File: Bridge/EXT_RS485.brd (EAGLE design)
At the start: 22.5 x 72 mm, 17 parts, among them IC1 SN65HVD72D, X1 V1, X2 GND, X3 V2, X4 TERM, X5 TERM

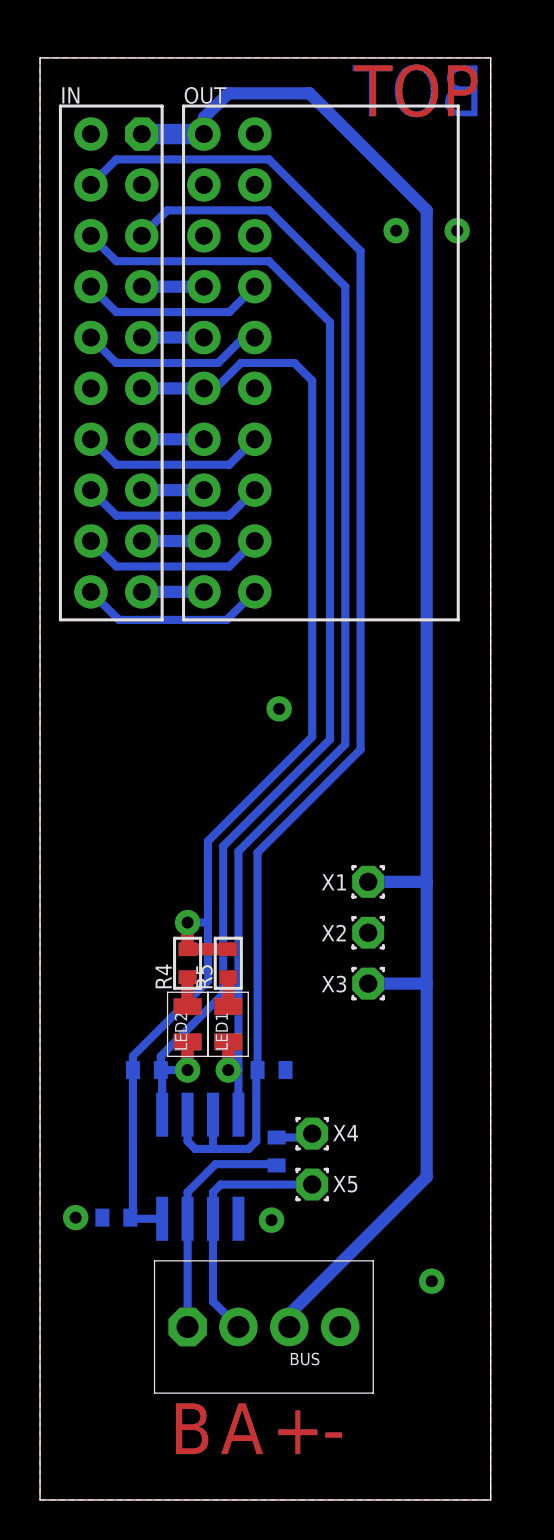
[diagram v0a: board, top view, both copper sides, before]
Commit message: Added S4M13
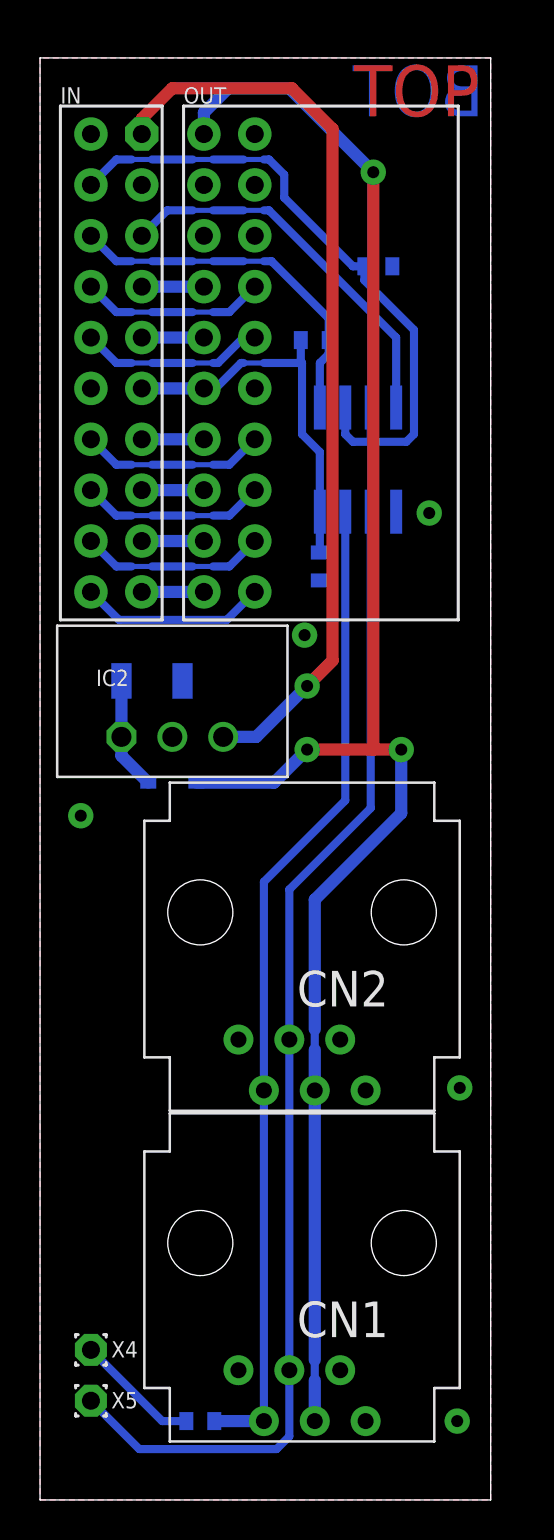
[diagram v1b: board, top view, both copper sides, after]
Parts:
- removed BUS: BUS, Conn:1725672
- removed LED1, LED2: (no value), Optic:0805
- removed R4, R5: 10k, RCL:0603
- removed X1: V1, Conn:T1.6/0.9
- removed X2: GND, Conn:T1.6/0.9
- removed X3: V2, Conn:T1.6/0.9
- added C2: nc, RCL:1206
- added CN1, CN2: RJ11, Conn:69254
- added D1: PMEG4005, Diode:SOD323
- added IC2: TSR 0.5-2450, DCDC:SIP3
- moved R1 40.5 mm to (16.9, 61.6)
- moved R3 37.4 mm to (13.7, 57.9)
- moved IC1 36.2 mm to (15.9, 51.9)
- moved C1 34.1 mm to (14.0, 46.6), turned to 90 degrees
- moved X4 15.4 mm to (2.54, 7.49)
- moved X5 15.4 mm to (2.54, 4.95)
- moved R2 14.0 mm to (8.00, 3.94), turned to 180 degrees
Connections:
- net N$13 renamed BUS-R
- removed net N$12: BUS.2, IC1.6, X5.1
- removed net N$14: LED2.C, R4.1
- removed net N$15: LED1.C, R5.1
- new net BUS-A: CN1.-3, CN2.-3, IC1.6, X5.1
- new net BUS-B: CN1.-2, CN2.-2, IC1.7, R2.2
- new net VOUT: IC2.P$3, IN.P$1
- net +3V3: no longer R4.2, R5.2
- net GND: now also C2.1, CN1.-5, CN2.-5, IC2.P$2; no longer BUS.4, X2.1
- net N$11: now also C2.2, D1.C, IC2.P$1; no longer BUS.1, IC1.7, R2.2
- net RX: no longer LED2.A
- net TX: no longer LED1.A
- net VIN: now also CN1.-4, CN2.-4, D1.A; no longer BUS.3, IN.P$1, X1.1, X3.1
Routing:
- net BUS-A: track 0.00 -> 59.0 mm
- net BUS-B: track 0.00 -> 49.6 mm
- net VOUT: track 0.00 -> 45.3 mm, vias 0 -> 1
- net +3V3: track 61.0 -> 19.5 mm, vias 1 -> 0
- net RX: track 59.6 -> 18.2 mm, vias 1 -> 0
- net TX: track 57.7 -> 19.4 mm, vias 1 -> 0
- net DE: track 69.3 -> 33.3 mm
- net N$12: track 12.4 -> 0.00 mm
- net N$11: track 11.8 -> 5.64 mm
- net VIN: track 82.4 -> 86.8 mm, vias 0 -> 3
- net BUS-R: track 1.86 -> 6.24 mm
- net N$15: track 1.47 -> 0.00 mm
- net N$14: track 1.47 -> 0.00 mm
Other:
- board text removed: "+"
- board text removed: "-"
- board text removed: "A"
- board text removed: "B"
